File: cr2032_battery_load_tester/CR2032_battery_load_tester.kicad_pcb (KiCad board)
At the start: 4 copper layers, 0 parts

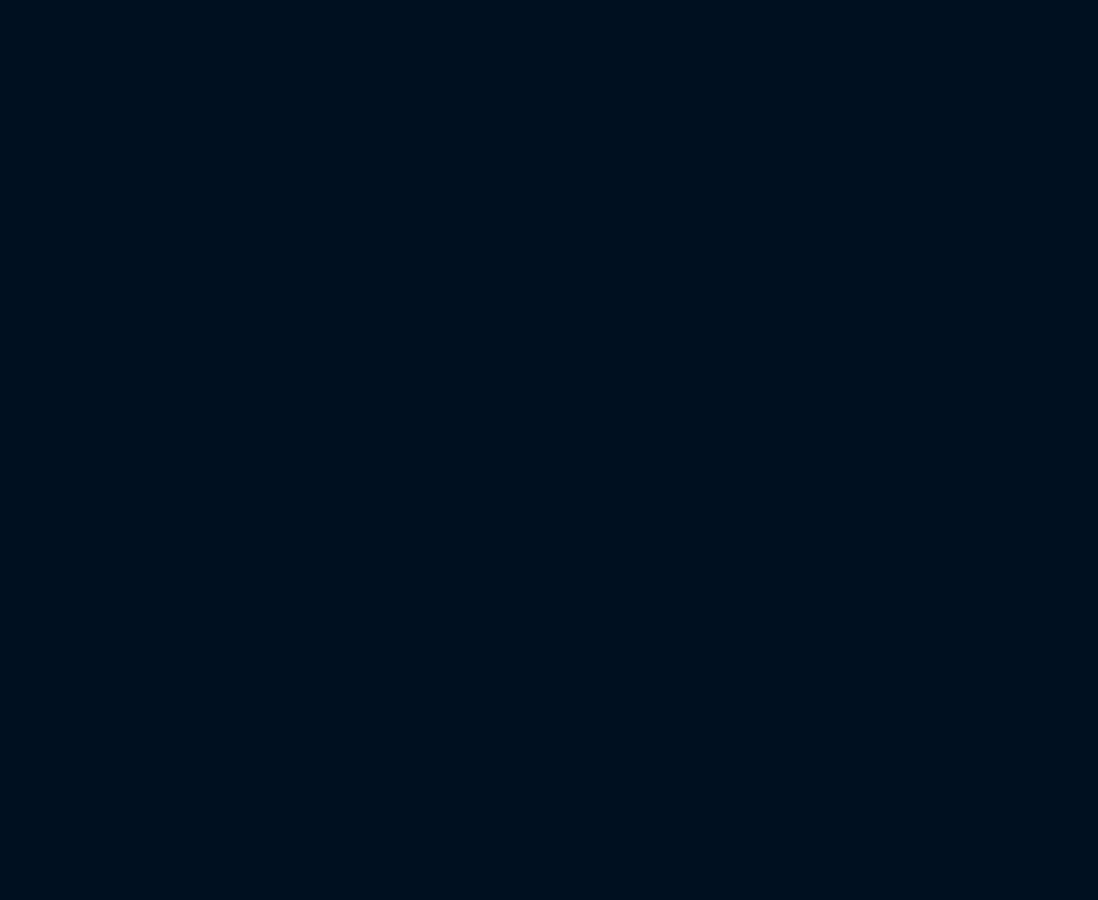
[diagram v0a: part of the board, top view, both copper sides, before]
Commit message: V1.0 of 2032 PCB
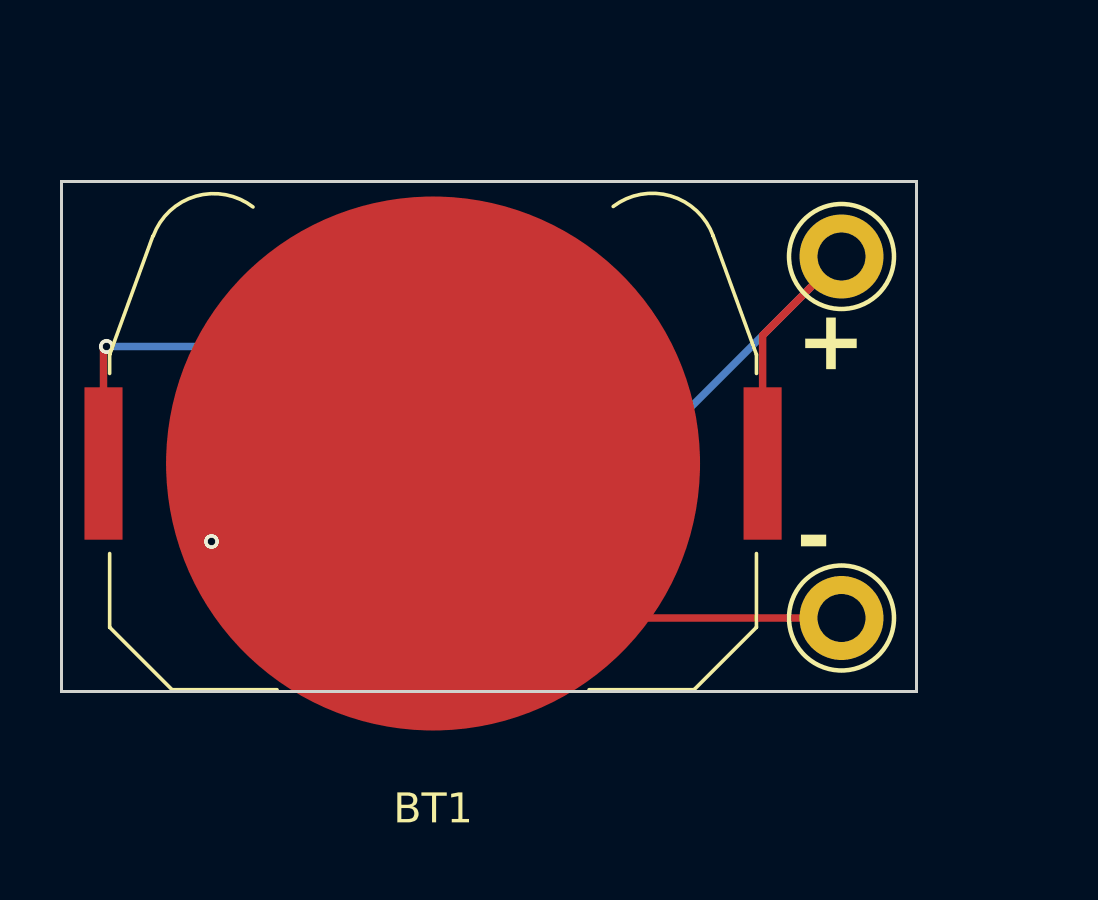
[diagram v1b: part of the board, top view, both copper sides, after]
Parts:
- added BT1: Battery_Cell, Battery:BatteryHolder_Keystone_3034_1x20mm, F.Cu at (62.4, 142.4)
- added R1: 100, Resistor_SMD:R_0603_1608Metric_Pad0.98x0.95mm_HandSolder, B.Cu at (68.0, 142.5)
- added SW1: SW_Push, Button_Switch_SMD:SW_Push_1P1T-SH_NO_CK_KMR2xxG, B.Cu at (55.5, 142.0)
- added TP1: TestPoint, TestPoint:TestPoint_Keystone_5010-5014_Multipurpose, F.Cu at (76.0, 135.5)
- added TP2: TestPoint, TestPoint:TestPoint_Keystone_5010-5014_Multipurpose, F.Cu at (76.0, 147.6)
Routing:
- net +BATT: track 0.00 -> 40.2 mm, vias 0 -> 1
- net GND: track 0.00 -> 29.4 mm, vias 0 -> 1
- net Net-(R1-Pad2): track 0.00 -> 16.1 mm
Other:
- board outline added: 28.5 x 17 mm
- copper layers 4 -> 2
- board text added: "+"
- board text added: "-"
- board text added: "SK Electronics 2032 Battery Load PCB 2023/11/13 V1.0"
- board text removed: "In1, [Description]"
- board text removed: "In2, [Description]"
